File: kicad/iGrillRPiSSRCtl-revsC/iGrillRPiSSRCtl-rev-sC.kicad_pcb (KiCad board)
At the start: 2 copper layers, 65 x 56 mm, 25 parts, among them J1 Screw_Terminal_01x02, P1 Conn_02x20_Odd_Even, Q1 Q_NPN_CBE, SW1 Off On

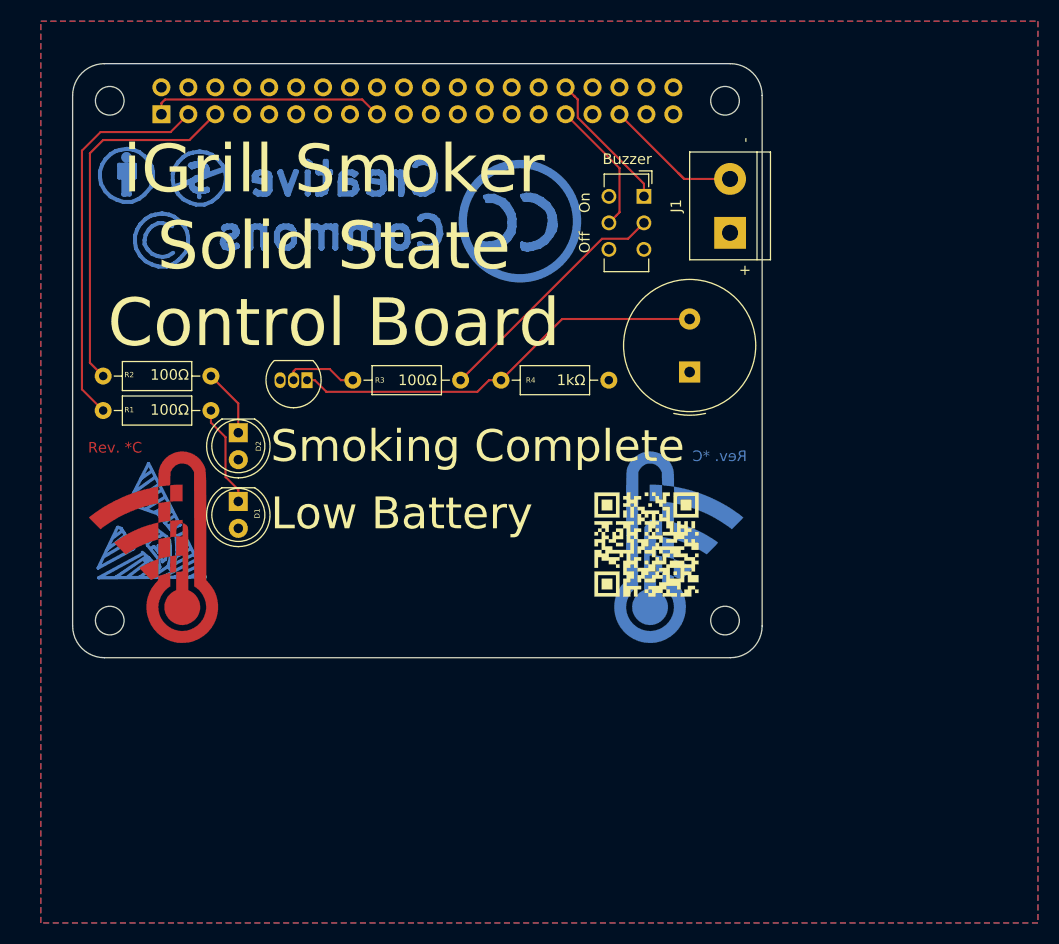
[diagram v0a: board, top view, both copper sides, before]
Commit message: Updates from protoype **
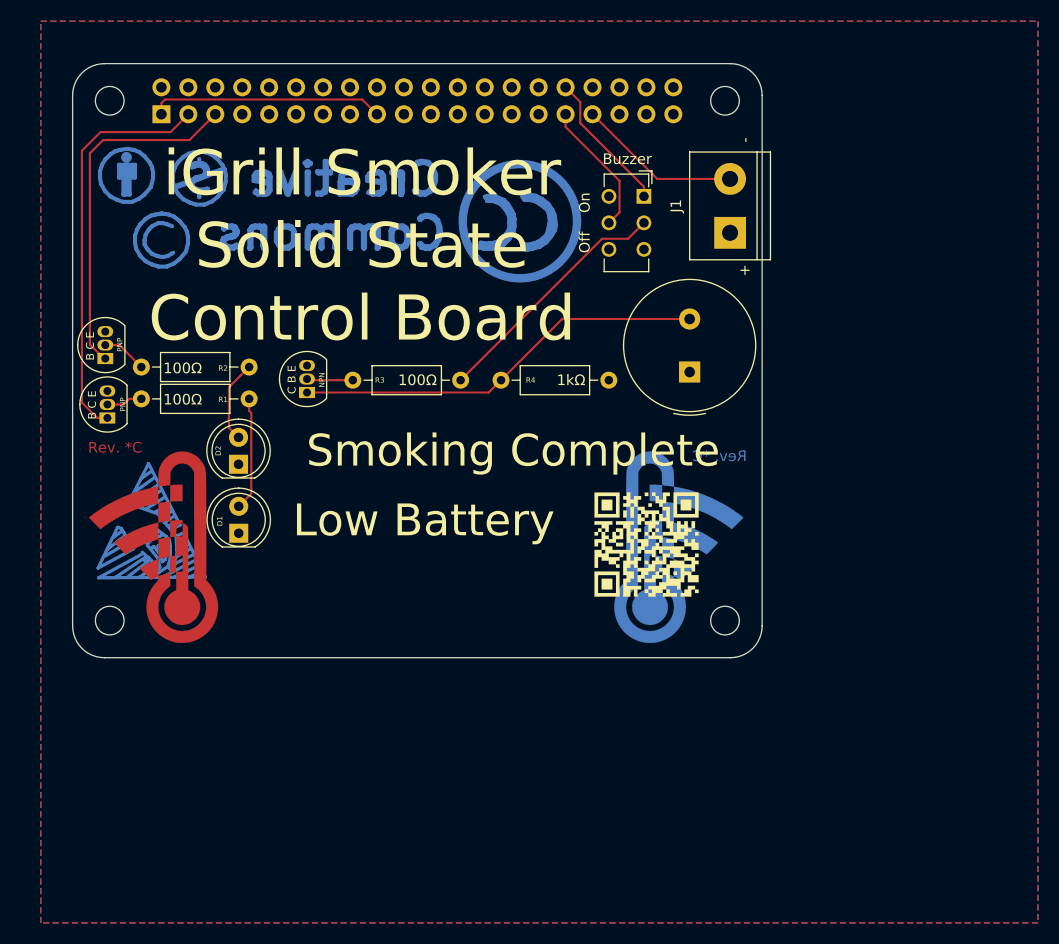
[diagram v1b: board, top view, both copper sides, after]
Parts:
- added Q2: Q_PNP_BCE, Package_TO_SOT_THT:TO-92_Inline, F.Cu at (20.4, 51.2)
- added Q3: Q_PNP_BCE, Package_TO_SOT_THT:TO-92_Inline, F.Cu at (20.2, 45.6)
- moved REF** 29.8 mm to (52.0, 56.6)
- moved G*** 13.9 mm to (62.0, 55.5)
- moved R1 13.8 mm to (33.8, 49.4), turned to 180 degrees
- moved R2 13.8 mm to (33.8, 46.4), turned to 180 degrees
- moved D1 3.00 mm to (32.8, 62.1), turned to 90 degrees
- moved D2 2.98 mm to (32.8, 55.6), turned to 90 degrees
- moved Q1 1.16 mm to (39.2, 48.8), turned to 90 degrees
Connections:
- D1 pad 1: Net-(D1-Pad1) -> GND
- D1 pad 2: +5V -> Net-(D1-Pad2)
- D2 pad 1: Net-(D2-Pad1) -> GND
- D2 pad 2: +5V -> Net-(D2-Pad2)
- J1 pad 2: /GPIO19(SPI1_MISO) -> /GPIO13(PWM1)
- R1 pad 1: /GPIO2(SDA1) -> Net-(D1-Pad2)
- R1 pad 2: Net-(D1-Pad1) -> Net-(Q2-Pad2)
- R2 pad 1: /GPIO3(SCL1) -> Net-(D2-Pad2)
- R2 pad 2: Net-(D2-Pad1) -> Net-(Q3-Pad2)
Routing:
- net /GPIO13(PWM1): track 0.00 -> 15.5 mm
- net /GPIO19(SPI1_MISO): track 13.7 -> 0.00 mm
- net Net-(D1-Pad2): track 0.00 -> 10.7 mm
- net Net-(D1-Pad1): track 9.64 -> 0.00 mm
- net Net-(D2-Pad2): track 0.00 -> 8.36 mm
- net Net-(D2-Pad1): track 6.98 -> 0.00 mm
- net Net-(Q3-Pad2): track 0.00 -> 4.26 mm
- net Net-(Q2-Pad2): track 0.00 -> 3.42 mm
- net Net-(Q1-Pad2): track 6.96 -> 4.36 mm
- net /GPIO3(SCL1): track 34.9 -> 33.4 mm
- net /GPIO2(SDA1): track 36.8 -> 38.2 mm
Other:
- board text added: "02 - Red LED 03 - Green LED 06 - Switch 12 - Buzzer 13 - SSR (J1)"
- board text added: "B C E"
- board text added: "BCM - Function"
- board text added: "C B E"
- board text added: "NPN"
- board text added: "PNP"
